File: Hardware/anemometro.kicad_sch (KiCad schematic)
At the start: 1 part, among them J31 R-RJ11R06P-A800

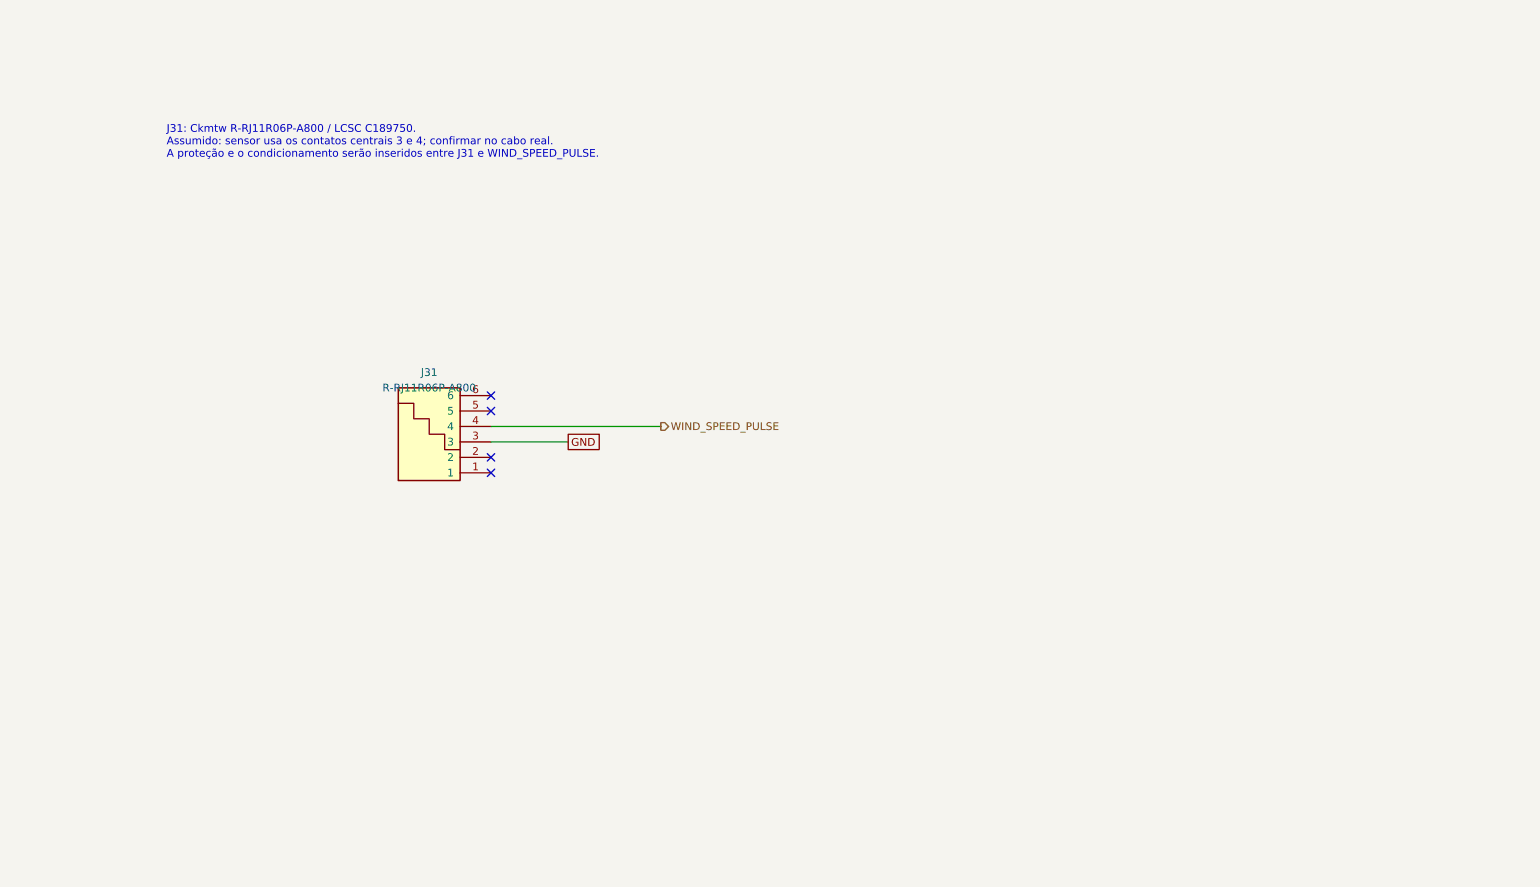
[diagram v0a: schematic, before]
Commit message: Sensores metereologicos -IA que fez
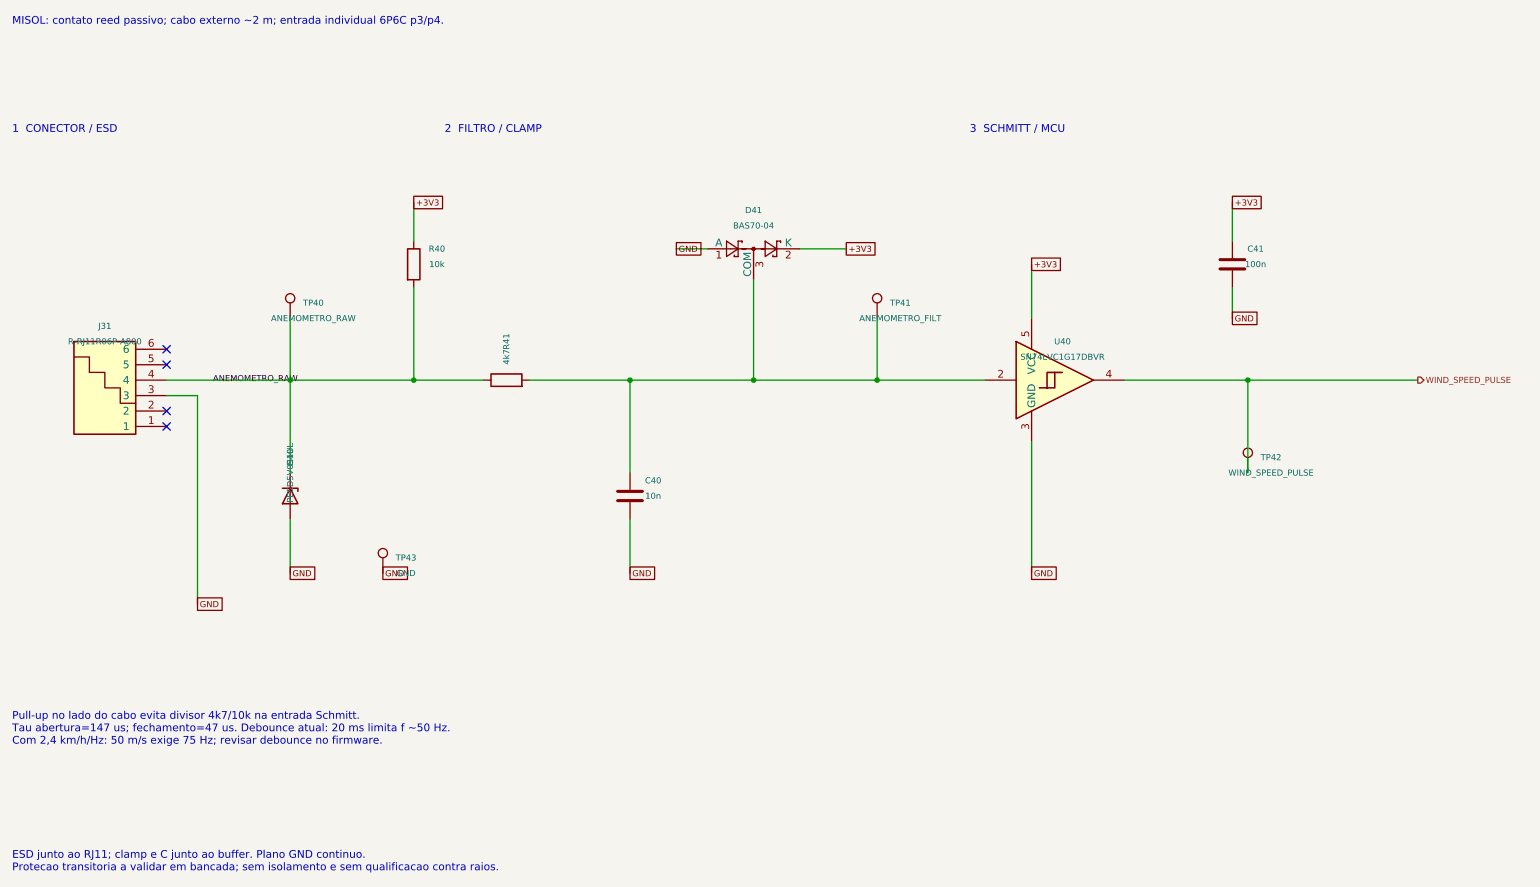
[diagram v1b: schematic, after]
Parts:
- added C40: 10n, Capacitor_SMD:C_0603_1608Metric, symbol Device:C
- added C41: 100n, Capacitor_SMD:C_0603_1608Metric, symbol Device:C
- added D40: PESD5V0S1UL, Diode_SMD:D_SOD-882, symbol Device:D_Zener
- added D41: BAS70-04, Package_TO_SOT_SMD:SOT-23, symbol Sensores_Meteo:BAS70-04
- added R40: 10k, Resistor_SMD:R_0603_1608Metric, symbol Device:R
- added R41: 4k7, Resistor_SMD:R_0603_1608Metric, symbol Device:R
- added TP40: ANEMOMETRO_RAW, TestPoint:TestPoint_Pad_D1.5mm, symbol Connector:TestPoint
- added TP41: ANEMOMETRO_FILT, TestPoint:TestPoint_Pad_D1.5mm, symbol Connector:TestPoint
- added TP42: WIND_SPEED_PULSE, TestPoint:TestPoint_Pad_D1.5mm, symbol Connector:TestPoint
- added TP43: GND, TestPoint:TestPoint_Pad_D1.5mm, symbol Connector:TestPoint
- added U40: SN74LVC1G17DBVR, Package_TO_SOT_SMD:SOT-23-5, symbol 74xGxx:74LVC1G17
- J31: Function (none) -> RJ11 individual; contatos centrais; LCSC (none) -> C189750; Manufacturer (none) -> Ckmtw; Rating (none) -> 6P6C; p3=return; p4=signal; THT
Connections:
- net GND: now also C40.2, C41.2, D40.2 (A), D41.1 (A), TP43.1, U40.3 (GND)
- net WIND_SPEED_PULSE: now also TP42.1, U40.4; no longer J31.4
- new net: C40.1, D41.3 (COM), R41.2, TP41.1, U40.2
- new net +3V3: C41.1, D41.2 (K), R40.1, U40.5 (VCC)
- new net ANEMOMETRO_RAW: D40.1 (K), J31.4, R40.2, R41.1, TP40.1
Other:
- note added: "1 CONECTOR / ESD"
- note added: "2 FILTRO / CLAMP"
- note added: "3 SCHMITT / MCU"
- note added: "ESD junto ao RJ11; clamp e C junto ao buffer. Plano GND continuo. Protecao transitoria a validar em bancada; sem isolamento e sem qualificacao contra raios."
- note added: "MISOL: contato reed passivo; cabo externo ~2 m; entrada individual 6P6C p3/p4."
- note added: "Pull-up no lado do cabo evita divisor 4k7/10k na entrada Schmitt. Tau abertura=147 us; fechamento=47 us. Debounce atual: 20 ms limita f ~50 Hz. Com 2,4 km/h/Hz: 50 m/s exige 75 Hz; revisar debounce no firmware."
- note removed: "J31: Ckmtw R-RJ11R06P-A800 / LCSC C189750. Assumido: sensor usa os contatos centrais 3 e 4; confirmar no cabo real. A proteção e o condicionamento serão inseridos entre J31 e WIND_SPEED_PULSE."
- company: (none) -> TCC - Estacao meteorologica
- title: (none) -> ANEMOMETRO - protecao e condicionamento
- moved on the sheet: J31

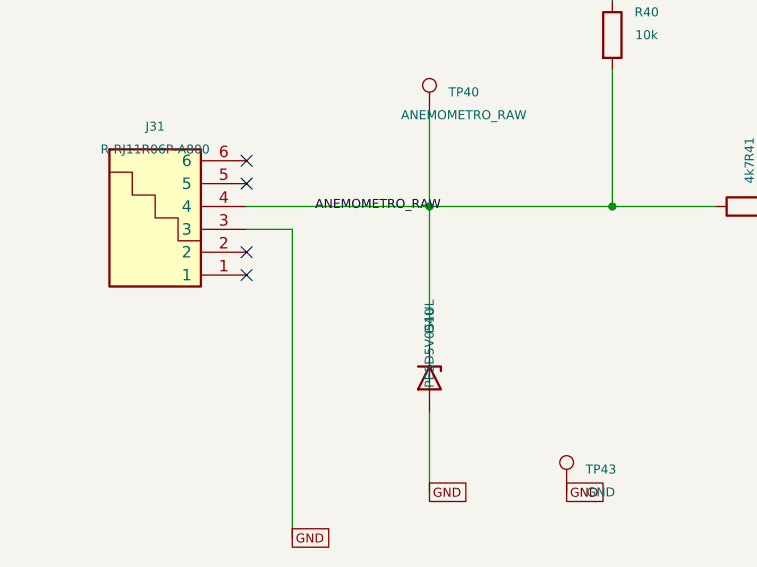
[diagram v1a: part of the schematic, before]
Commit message: design sensores pronto
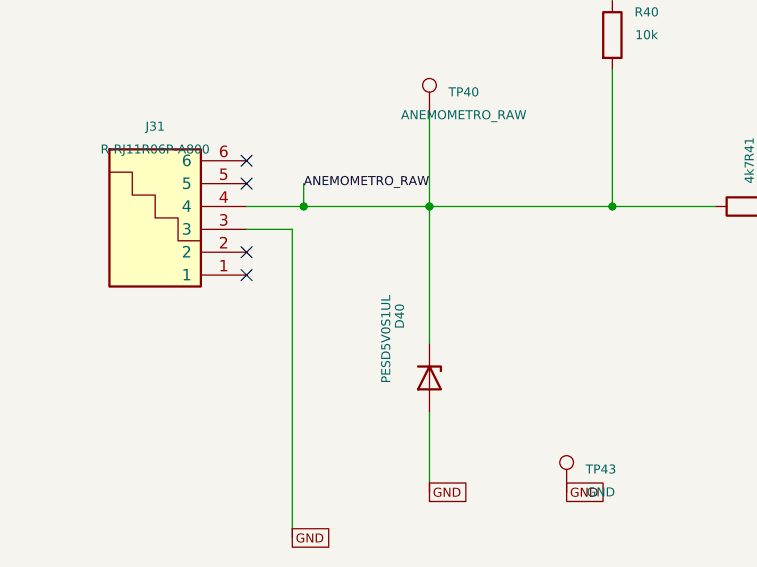
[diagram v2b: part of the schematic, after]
